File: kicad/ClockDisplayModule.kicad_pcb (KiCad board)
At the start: 2 copper layers, 88.9 x 33 mm, 13 parts, among them P101 CONN_01X05, U101 MAX7221

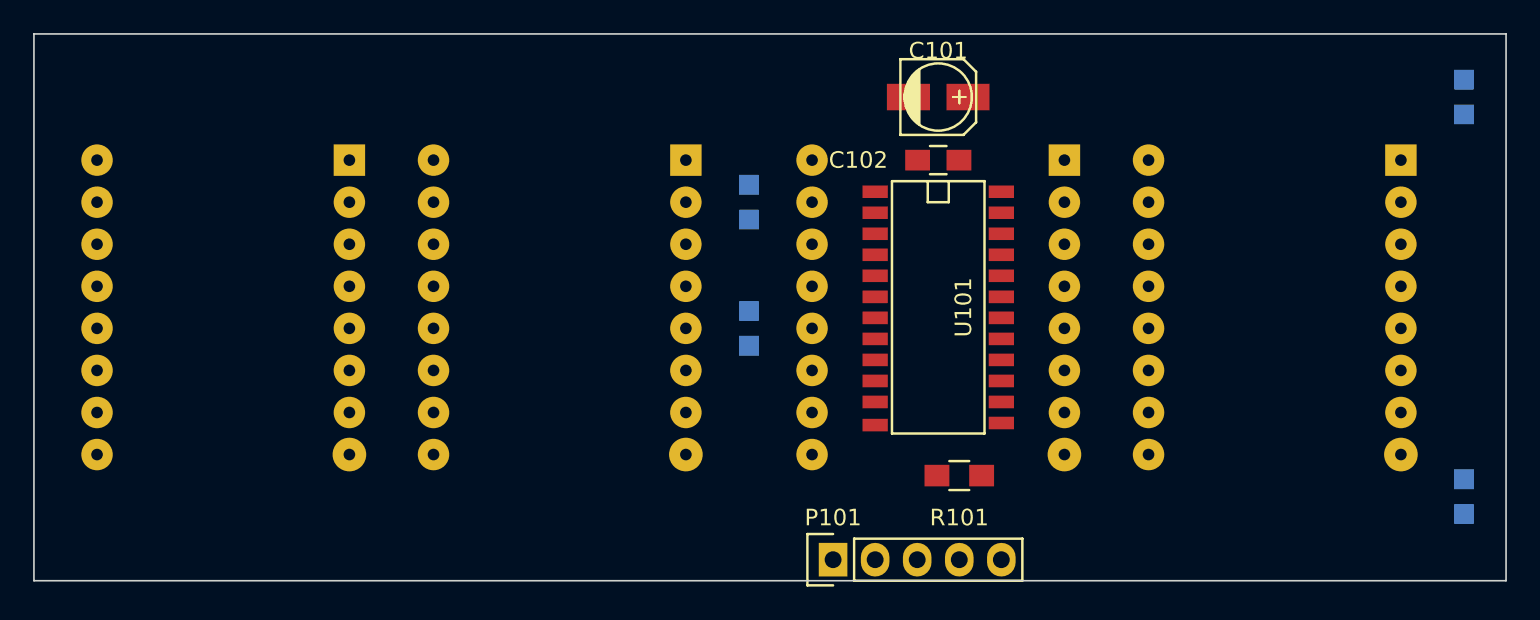
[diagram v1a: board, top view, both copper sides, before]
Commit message: Initial layout before routing
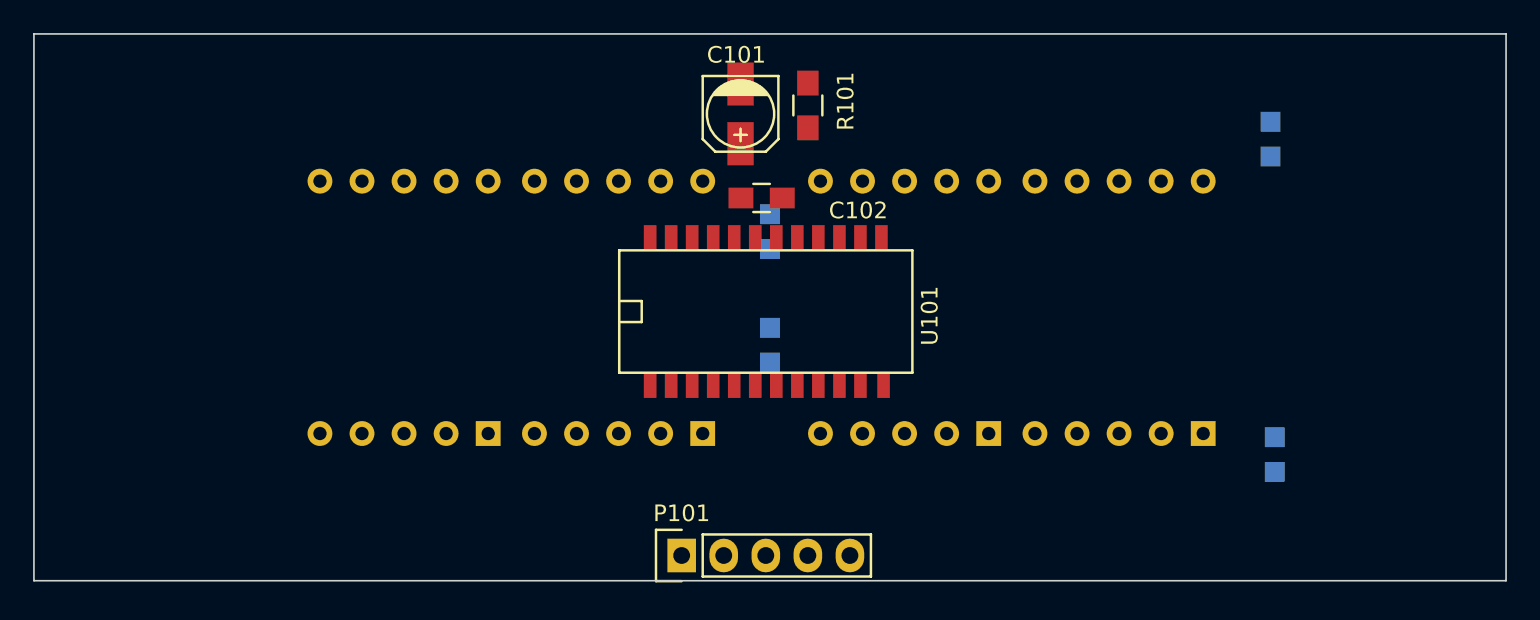
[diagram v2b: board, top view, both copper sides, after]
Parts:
- AFF101, AFF102, AFF103, AFF104: value 7SEGMENTS-CC -> NKR161B; footprint ClockFootprints:SC08-11SURKWA -> ClockFootprints:161_163_Series
- U101: footprint SMD_Packages:SOIC-24 -> ClockFootprints:SOIC-24
- moved R101 24.2 mm to (117.9, 39.9), turned to 90 degrees
- moved C101 12.0 mm to (113.8, 40.4), turned to 270 degrees
- moved D104 12.0 mm to (145.8, 41.9)
- moved D103 11.7 mm to (146.1, 61.0)
- moved AFF104 10.9 mm to (93.5, 52.1)
- moved C102 10.9 mm to (115.1, 45.5), turned to 0 degrees
- moved U101 10.4 mm to (115.3, 52.3), turned to 0 degrees
- moved AFF101 9.40 mm to (136.7, 52.1)
- moved P101 9.15 mm to (110.2, 67.1)
- moved AFF103 3.56 mm to (106.4, 52.1)
- moved D101 2.18 mm to (115.6, 47.5)
- moved AFF102 2.03 mm to (123.7, 52.1)
- moved D102 1.63 mm to (115.6, 54.4)
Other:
- net class Default: clearance 0.2 -> 0.254; trace_width 0.25 -> 0.254; via_dia 0.6 -> 0.6858; via_drill 0.4 -> 0.3302
- rule trace_clearance: 0.2 -> 0.254
- rule trace_min: 0.2 -> 0.1524
- rule via_min_drill: 0.3 -> 0.3302
- rule via_min_size: 0.4 -> 0.6858
